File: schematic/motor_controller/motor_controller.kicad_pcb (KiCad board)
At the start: 2 copper layers, 53.5 x 34.1 mm, 22 parts, among them J1 Micro_SD_Card, J2 Conn_01x20_Pin, J3 Conn_01x01_Pin, J4 Conn_01x20_Pin, U1 AMS1117-5.0, U2 74LVC125APW_118, U3 LM386

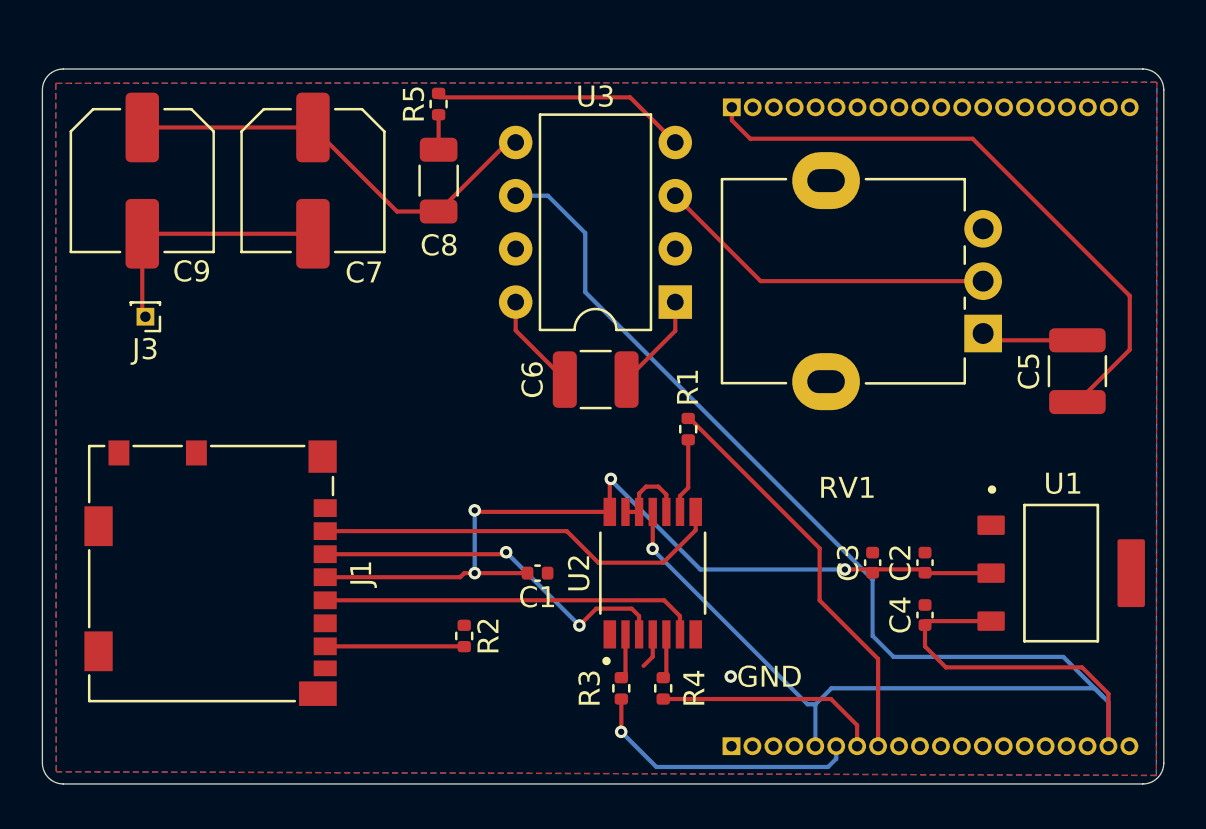
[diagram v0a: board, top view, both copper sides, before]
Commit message: Final schematic reviewed
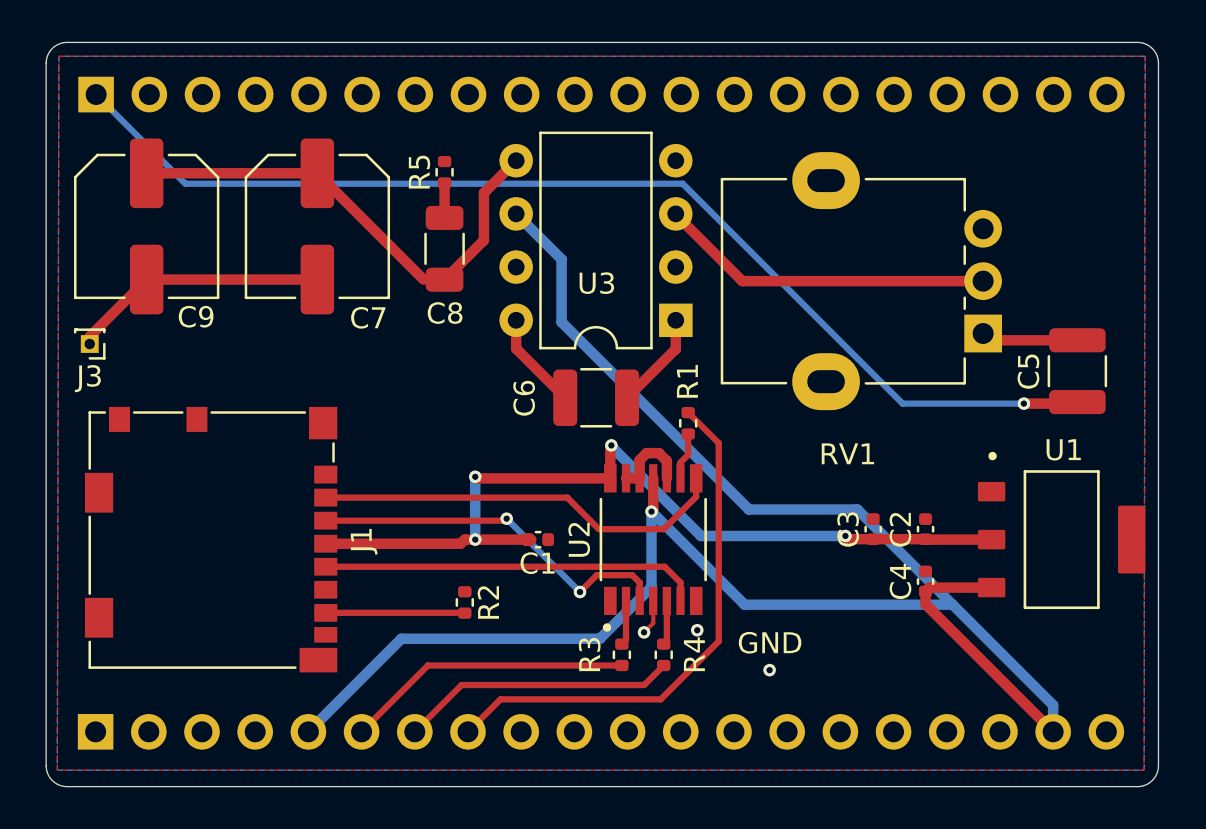
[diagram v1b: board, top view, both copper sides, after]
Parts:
- J2, J4: footprint Connector_PinHeader_1.00mm:PinHeader_1x20_P1.00mm_Vertical -> Connector_PinHeader_2.54mm:PinHeader_1x20_P2.54mm_Vertical
- moved J4 30.4 mm to (85.6, 67.3)
- moved J2 30.4 mm to (85.6, 36.9)
- moved C8 3.27 mm to (102.3, 44.3)
- moved R5 3.27 mm to (102.3, 40.6)
- moved J3 2.96 mm to (85.3, 48.8)
- moved C7 2.20 mm to (96.2, 43.2)
- moved C9 2.20 mm to (88.1, 43.2)
- moved C1 1.60 mm to (106.7, 58.1)
- moved C2 1.60 mm to (125.2, 57.6)
- moved C3 1.60 mm to (122.7, 57.6)
- moved C4 1.60 mm to (125.2, 60.1)
- moved J1 1.60 mm to (91.2, 58.1)
- moved R2 1.60 mm to (103.2, 61.1)
- moved R3 1.60 mm to (110.7, 63.6)
- moved R4 1.60 mm to (112.7, 63.6)
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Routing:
- net /Audio: track 29.2 -> 53.0 mm, vias 0 -> 1
- net GND: track 17.9 -> 5.66 mm, vias 1 -> 3
- net /CS: track 19.6 -> 25.3 mm
- net +5V: track 89.1 -> 91.5 mm
- net /SCK: track 10.8 -> 13.2 mm
- net Net-(C7-Pad1): track 21.9 -> 23.4 mm
- net Net-(U2-3A): track 3.60 -> 2.27 mm
- net /MOSI: track 13.3 -> 13.7 mm, vias 1 -> 0
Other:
- board size 53.5 x 34.1 mm -> 53.1 x 35.5 mm
